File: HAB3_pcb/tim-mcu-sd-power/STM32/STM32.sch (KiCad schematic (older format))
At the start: 40 parts, among them J1 Conn_ARM_JTAG_SWD_20, J2 Micro_SD_Card_Det, J3 Conn_01x16_Male, J4 Conn_01x16_Male, J5 Conn_01x16_Male, J6 Conn_01x02_Male, J7 Conn_01x02_Male, J8 Conn_01x02_Male, J9 Conn_01x11_Male, SW1 SW_DPST_x2, U1 STM32F401RET6, U2 LD3985M33R_SOT23, Y1 32.768MHz

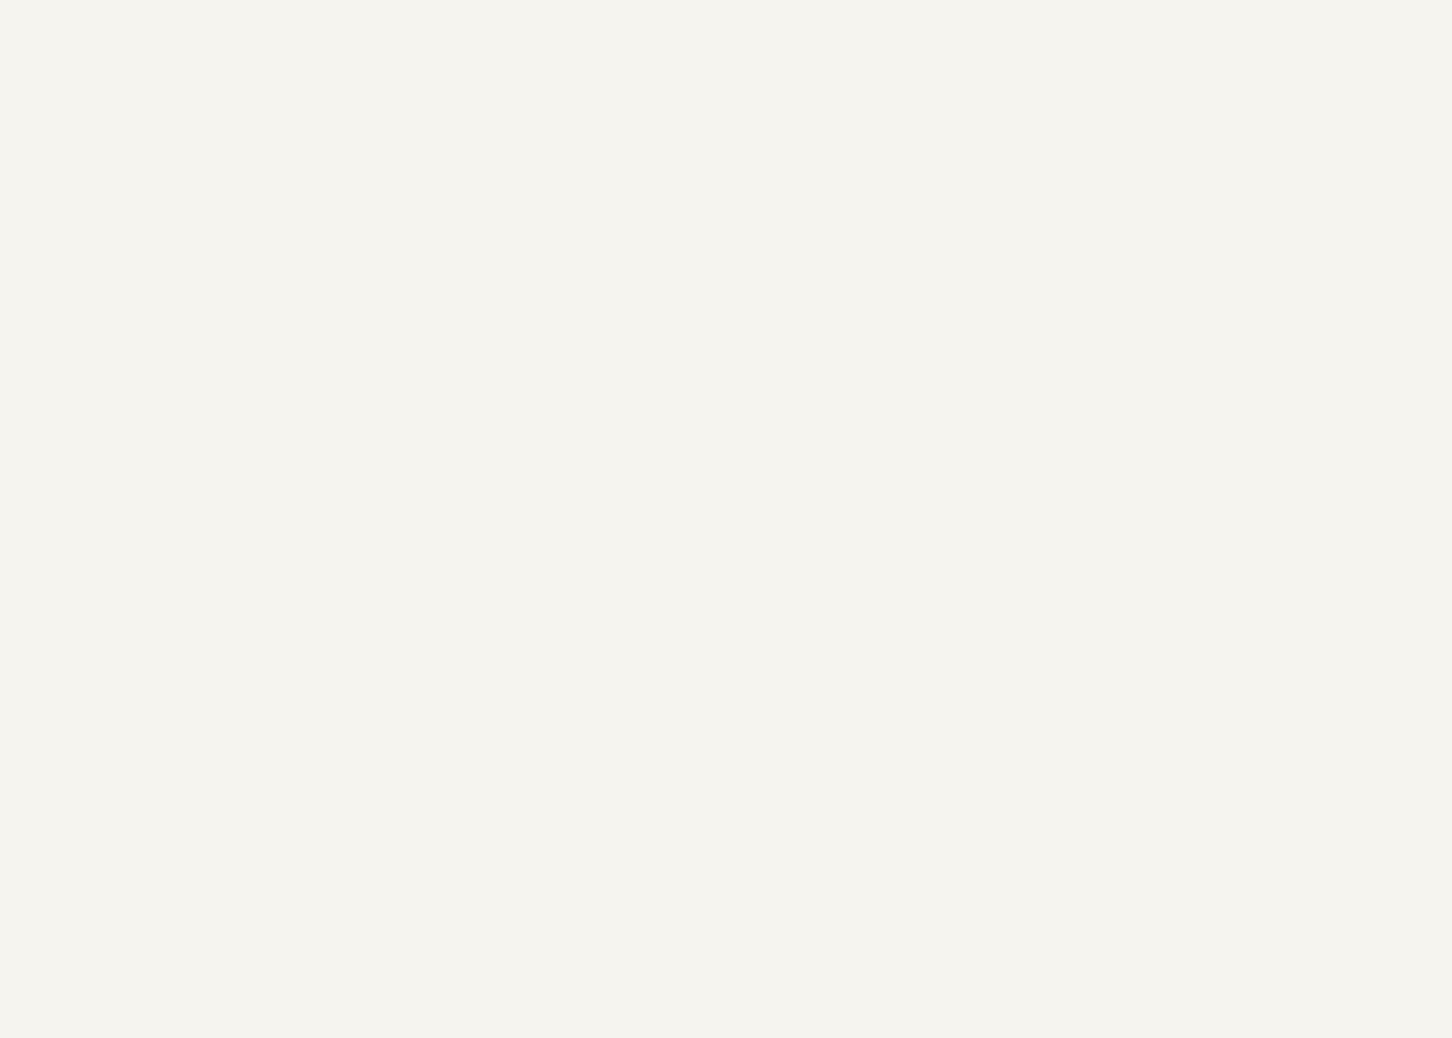
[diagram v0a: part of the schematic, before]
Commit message: halfway done with  power regulator
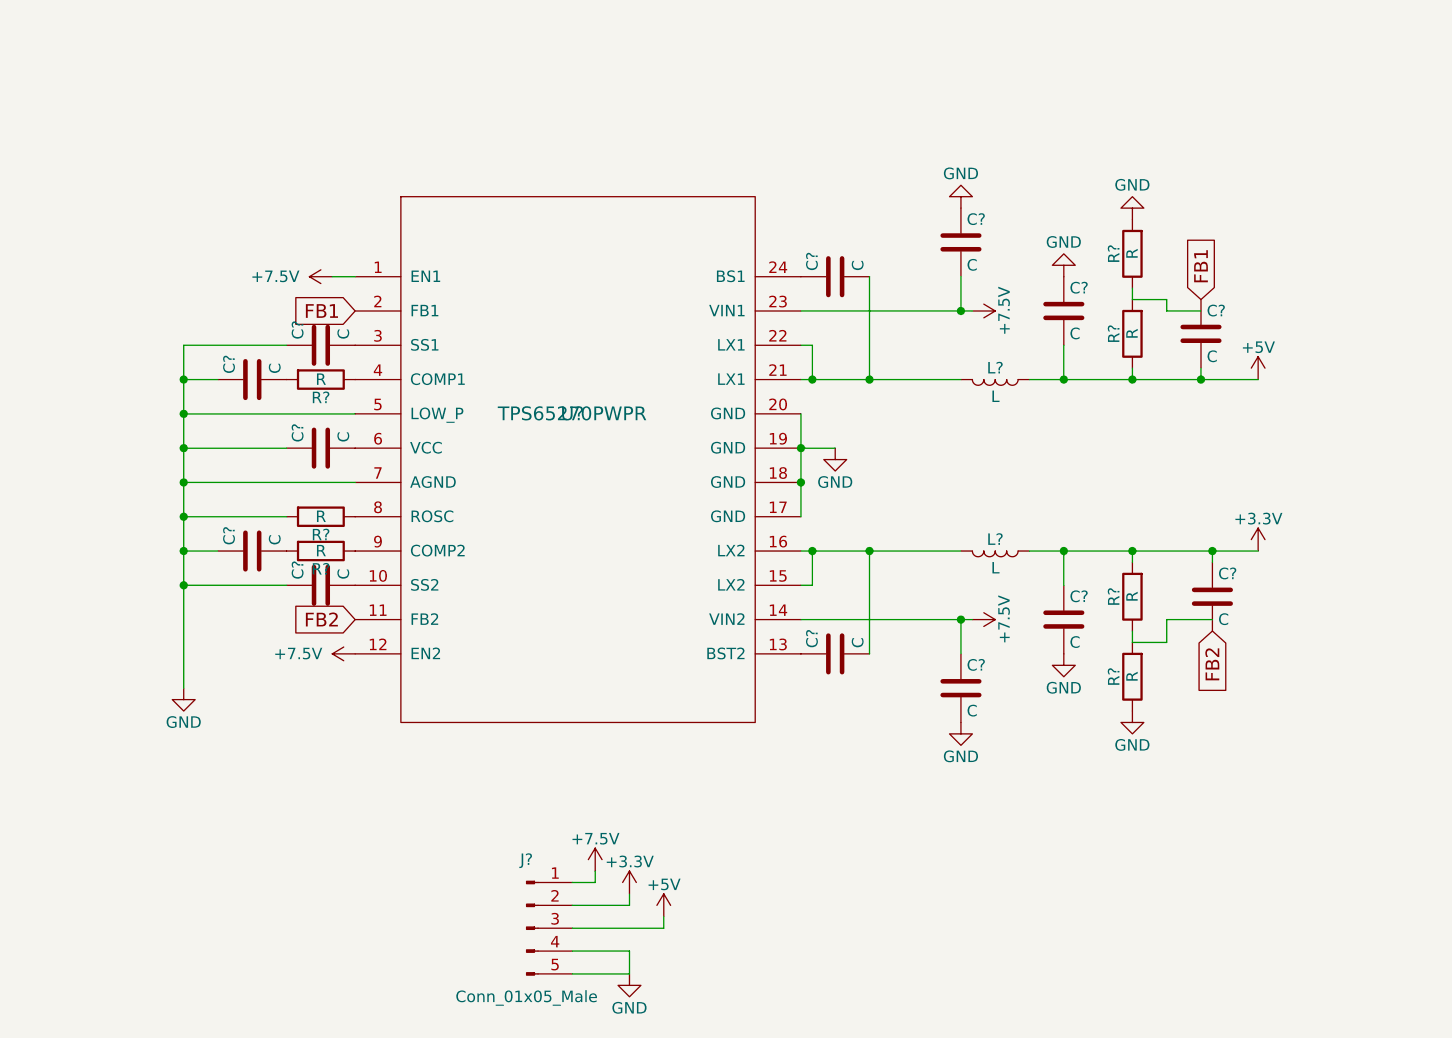
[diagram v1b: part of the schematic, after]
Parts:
- added C? (x13): C, symbol C
- added J?: Conn_01x05_Male, symbol Conn_01x05_Male
- added L? (x2): L, symbol L
- added R? (x7): R, symbol R
- added U?: TPS65270PWPR, symbol TPS65270PWPR
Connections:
- net +3V3: now also C?.1, C?.1, J?.2 (Pin_2), L?.1, R?.2
- net GND: now also C?.1, C?.1, C?.1, C?.1, C?.1, C?.1, C?.1, C?.2, C?.2, J?.4 (Pin_4), J?.5 (Pin_5), R?.1, R?.2, R?.2, U?.17 (GND), U?.18 (GND), U?.19 (GND), U?.20 (GND), U?.5 (LOW_P), U?.7 (AGND)
- new net: C?.2, U?.10 (SS2)
- new net: C?.1, U?.13 (BST2)
- new net: C?.2, L?.2, U?.15 (LX2), U?.16 (LX2)
- new net: C?.2, L?.2, U?.21 (LX1), U?.22 (LX1)
- new net: C?.1, U?.24 (BS1)
- new net: C?.2, U?.3 (SS1)
- new net: R?.1, U?.4 (COMP1)
- new net: C?.2, U?.6 (VCC)
- new net: R?.1, U?.8 (ROSC)
- new net: R?.1, U?.9 (COMP2)
- new net: C?.2, R?.2 (x2)
- new net: R?.1, R?.2 (x2)
- new net +5V: C?.2, C?.2, J?.3 (Pin_3), L?.1, R?.1
- new net +7.5V: C?.1, C?.2, J?.1 (Pin_1), U?.1 (EN1), U?.12 (EN2), U?.14 (VIN2), U?.23 (VIN1)
- new net FB1: C?.1, U?.2 (FB1)
- new net FB2: C?.2, U?.11 (FB2)
